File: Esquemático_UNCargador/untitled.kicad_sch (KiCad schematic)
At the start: 13 parts, among them U3.3 LM2596S-3.3, U5 LM2596S-5

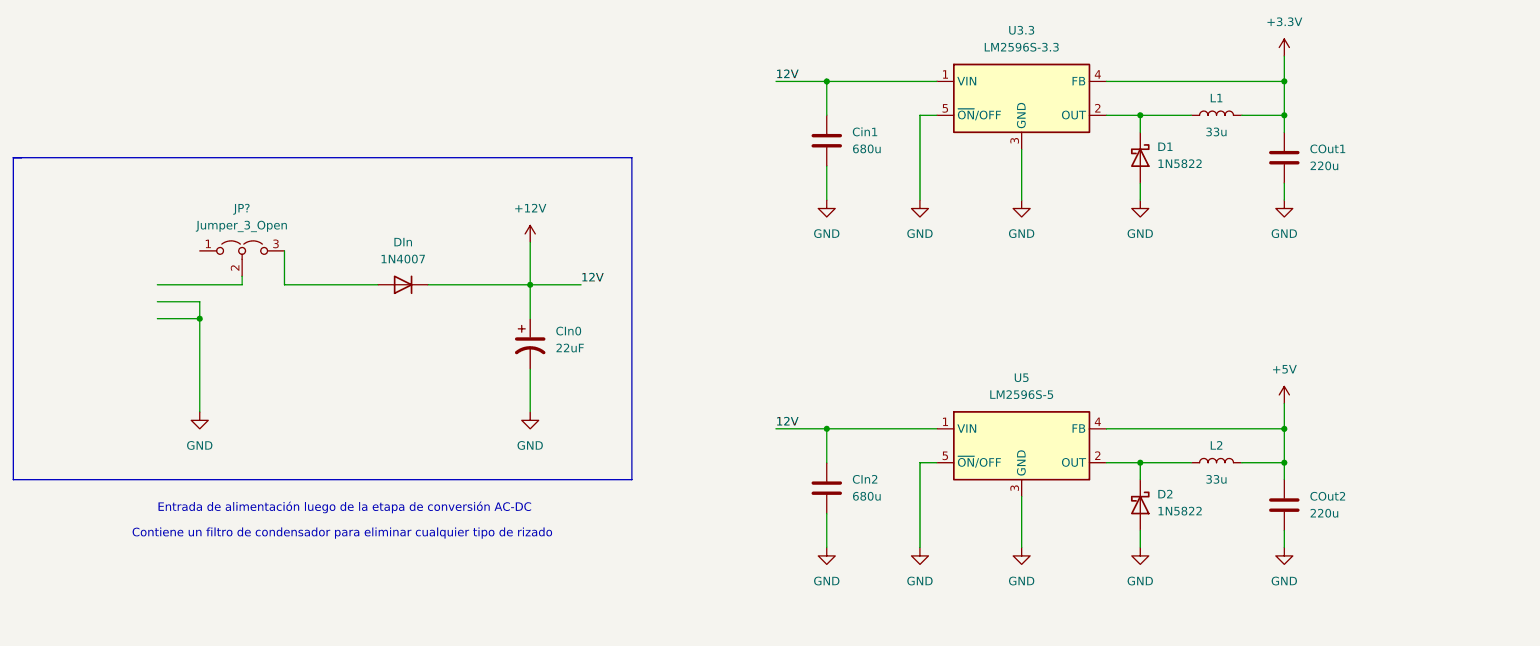
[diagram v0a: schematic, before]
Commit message: Actualizacion 23-03-23
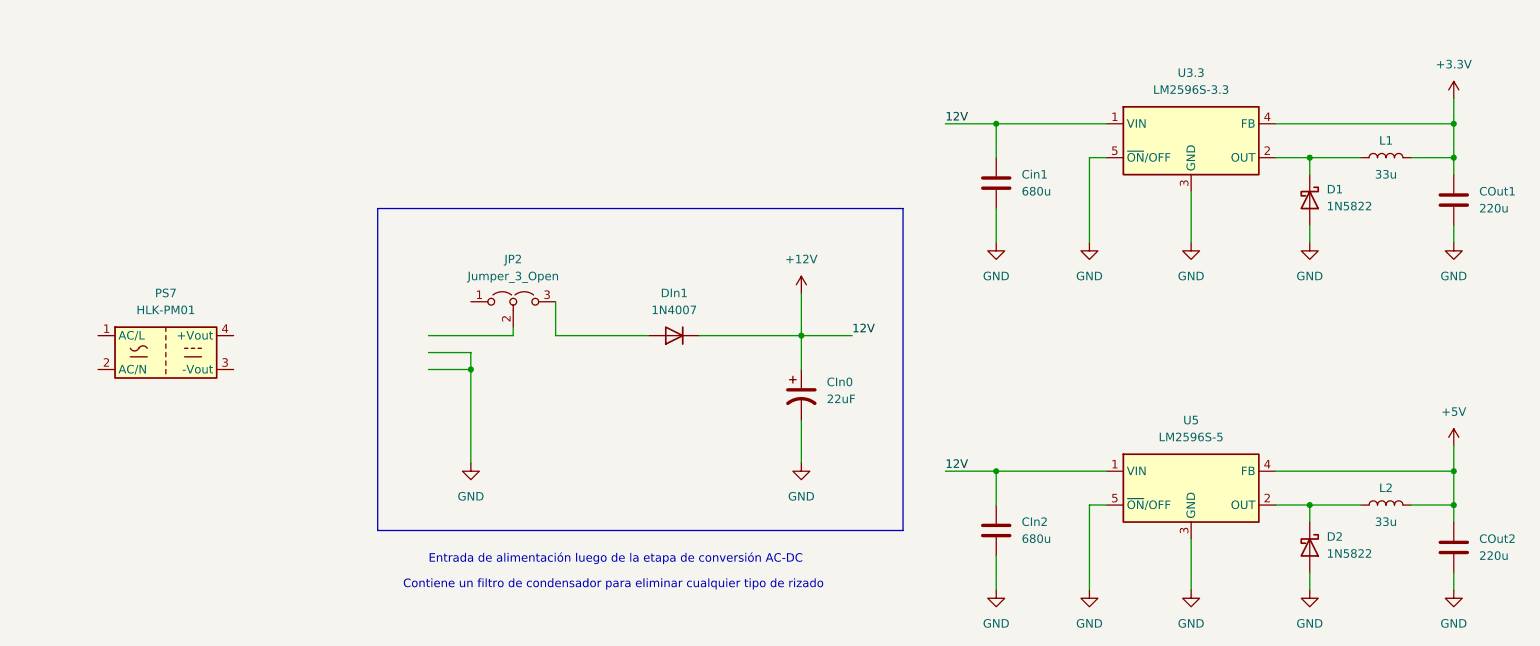
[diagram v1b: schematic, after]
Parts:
- added PS7: HLK-PM01, Convertidor_AC-DC:AC-DC_Converter, symbol Converter_ACDC:HLK-PM01
- CIn2, COut1, COut2: footprint (none) -> Capacitor_SMD:C_0201_0603Metric
- Cin1: footprint (none) -> Capacitor_SMD:C_0805_2012Metric_Pad1.18x1.45mm_HandSolder
- L1, L2: footprint (none) -> Inductor_SMD:L_Coilcraft_XxL4040
- gave numbers to parts that had none: 1
- renumbered DIn to DIn1
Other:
- moved on the sheet: CIn0, CIn2, COut1, COut2, Cin1, D1, D2, DIn1, JP2, L1, L2, U3.3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
